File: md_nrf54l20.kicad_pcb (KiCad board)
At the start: 4 copper layers, 68.6 x 53.3 mm, 46 parts, among them J1 POWER, J2 DIGITAL_8_13, J3 ANALOG, J4 DIGITAL_0_7, J5 USB_C, J6 USB_C, J7 Conn_01x04, SW1 RESET, U1 nRF54L20, U2 AMS1117-3.3, U3 CH347T, Y1 8MHz, Y2 32MHz

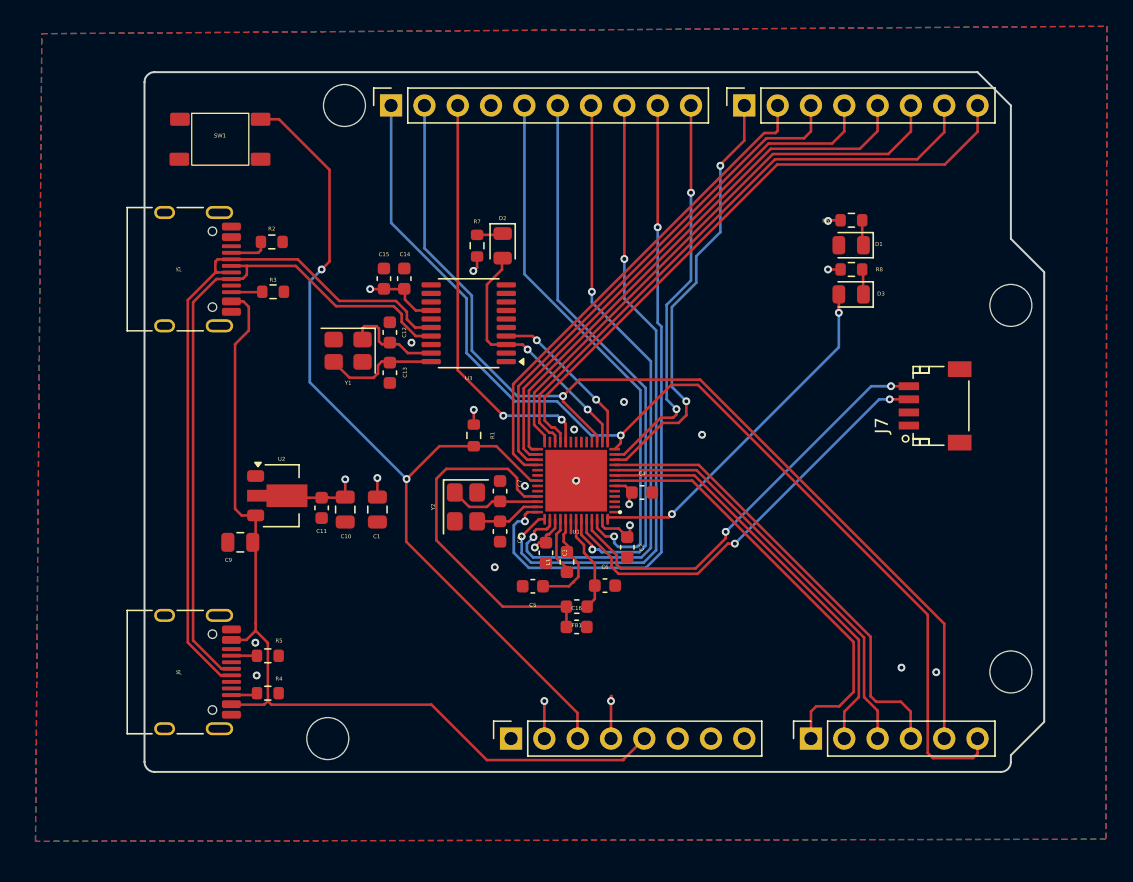
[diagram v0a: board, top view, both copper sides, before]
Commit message: Update layout
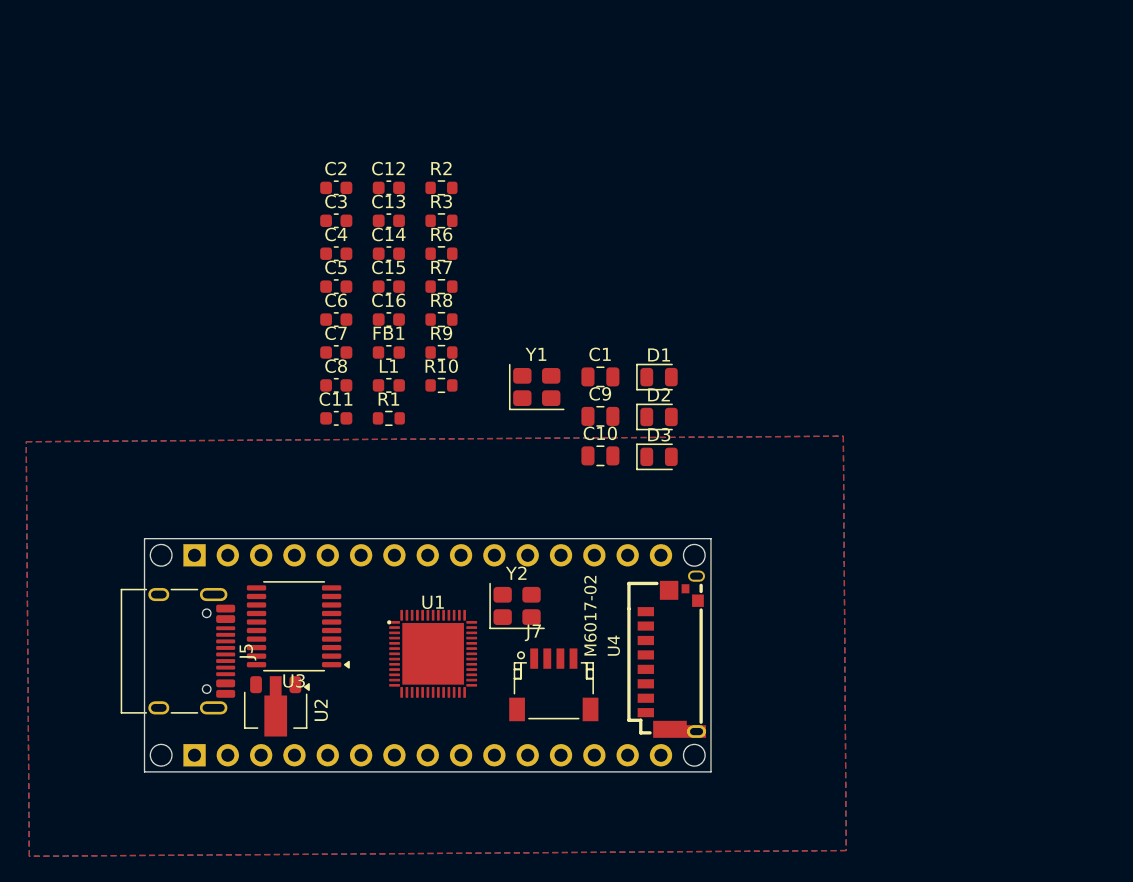
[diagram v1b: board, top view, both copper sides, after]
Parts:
- removed J1: POWER, Connector_PinSocket_2.54mm:PinSocket_1x08_P2.54mm_Vertical
- removed J2: DIGITAL_8_13, Connector_PinSocket_2.54mm:PinSocket_1x10_P2.54mm_Vertical
- removed J3: ANALOG, Connector_PinSocket_2.54mm:PinSocket_1x06_P2.54mm_Vertical
- removed J4: DIGITAL_0_7, Connector_PinSocket_2.54mm:PinSocket_1x08_P2.54mm_Vertical
- removed J6: USB_C, Connector_USB:USB_C_Receptacle_HRO_TYPE-C-31-M-12
- removed R4, R5: 5.1k, Resistor_SMD:R_0603_1608Metric
- removed SW1: RESET, md_nrf54l20:micro-switch
- added J10: Conn_01x15, Connector_PinHeader_2.54mm:PinHeader_1x15_P2.54mm_Vertical, B.Cu at (103.8, 83.5)
- added J9: Conn_01x15, Connector_PinHeader_2.54mm:PinHeader_1x15_P2.54mm_Vertical, B.Cu at (103.8, 98.7)
- added R10: 10k, Resistor_SMD:R_0603_1608Metric, F.Cu at (122.6, 70.5)
- added R9: 10k, Resistor_SMD:R_0603_1608Metric, F.Cu at (122.6, 68.0)
- added U4: M6017-02, md_nrf54l20:SIM-SMD_M6017-02, F.Cu at (140.2, 91.0)
- MH1, MH2, MH3, MH4: value MountingHole_3.2mm -> MountingHole_65mil; footprint Arduino_MountingHole:MountingHole_3.2mm -> Arduino_MountingHole:MountingHole_65mil
- moved MH1 51.5 mm to (101.3, 98.7)
- moved J7 35.9 mm to (131.2, 93.3), turned to 0 degrees
- moved C2 35.3 mm to (114.6, 55.5), turned to 0 degrees
- moved R8 31.5 mm to (122.6, 65.5), turned to 0 degrees
- moved R6 31.4 mm to (122.6, 60.5)
- moved MH3 30.7 mm to (141.9, 83.5)
- moved C3 29.9 mm to (114.6, 58.0), turned to 0 degrees
- moved C4 29.6 mm to (114.6, 60.5)
- moved J5 29.1 mm to (102.1, 90.8)
- moved C9 29.1 mm to (134.8, 72.9), turned to 0 degrees
- moved C6 28.8 mm to (114.6, 65.5)
- moved C16 27.5 mm to (118.6, 65.5)
- moved C5 27.3 mm to (114.6, 63.0), turned to 0 degrees
- moved U3 26.7 mm to (111.4, 88.9)
- moved MH4 25.0 mm to (141.9, 98.7)
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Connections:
- J7 pad 1: unconnected-(J7-Pin_1-Pad1) -> GND
- J7 pad 2: unconnected-(J7-Pin_2-Pad2) -> +3V3
- J7 pad 3: Net-(J7-Pin_3) -> unconnected-(J7-Pin_3-Pad3)
- J7 pad 4: Net-(J7-Pin_4) -> unconnected-(J7-Pin_4-Pad4)
- U1 pad 11: /D7 -> /A1
- U1 pad 12: /D8 -> /A2
- U1 pad 13: /A5_SCL -> /A3
- U1 pad 16: /A4_SDA -> unconnected-(U1-P1.06-Pad16)
- U1 pad 22: /AREF -> unconnected-(U1-P1.07-Pad22)
- U1 pad 23: /D0_RX -> unconnected-(U1-P1.08-Pad23)
- U1 pad 24: /D1_TX -> unconnected-(U1-P1.09-Pad24)
- U1 pad 39: /D9_PWM -> unconnected-(U1-P1.15-Pad39)
- U1 pad 40: /D10_CS -> unconnected-(U1-P1.16-Pad40)
- U1 pad 41: /D11_COTI -> unconnected-(U1-P1.18-Pad41)
- U1 pad 47: /D12_CITO -> unconnected-(U1-P1.19-Pad47)
- U1 pad 48: Net-(J7-Pin_3) -> unconnected-(U1-P1.20-Pad48)
- U1 pad 49: Net-(J7-Pin_4) -> unconnected-(U1-P1.21-Pad49)
- U1 pad 50: /D13_SCK -> unconnected-(U1-P1.24-Pad50)
- U1 pad 7: /A0 -> unconnected-(U1-P1.29-Pad7)
- U1 pad 8: /A1 -> unconnected-(U1-P1.30-Pad8)
- U1 pad 9: /A2 -> unconnected-(U1-P1.31-Pad9)
- U3 pad 10: unconnected-(U3-DTR1/MODE0-Pad10) -> /MODE_D
- U3 pad 13: unconnected-(U3-RTS1/MODE1-Pad13) -> /MODE_R
- U3 pad 5: unconnected-(U3-SCS0/TMS-Pad5) -> /SWDIO
- U3 pad 6: unconnected-(U3-SCK/TCK-Pad6) -> /SWDCLK
- U3 pad 9: unconnected-(U3-SCS1/TRST-Pad9) -> /nRESET
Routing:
- net /A5_SCL: track 84.9 -> 0.00 mm, vias 1 -> 0
- net /A4_SDA: track 79.2 -> 0.00 mm, vias 1 -> 0
- net /nRESET: track 71.3 -> 0.00 mm, vias 2 -> 0
- net VBUS: track 70.0 -> 0.00 mm
- net /USB_DN: track 54.5 -> 0.00 mm
- net /USB_DP: track 53.0 -> 0.00 mm
- net /D9_PWM: track 51.0 -> 0.00 mm, vias 2 -> 0
- net /D10_CS: track 49.4 -> 0.00 mm, vias 2 -> 0
- net /D11_COTI: track 49.2 -> 0.00 mm, vias 2 -> 0
- net /D0_RX: track 47.4 -> 0.00 mm
- net /D1_TX: track 45.4 -> 0.00 mm
- net /D12_CITO: track 43.3 -> 0.00 mm, vias 1 -> 0
- net /D2: track 43.0 -> 0.00 mm
- net /D13_SCK: track 42.2 -> 0.00 mm, vias 1 -> 0
- net /D3_PWM: track 41.7 -> 0.00 mm
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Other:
- board size 68.6 x 53.3 mm -> 43.2 x 17.8 mm
- board text added: "USB-C"
